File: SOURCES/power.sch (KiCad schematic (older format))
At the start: 1 part

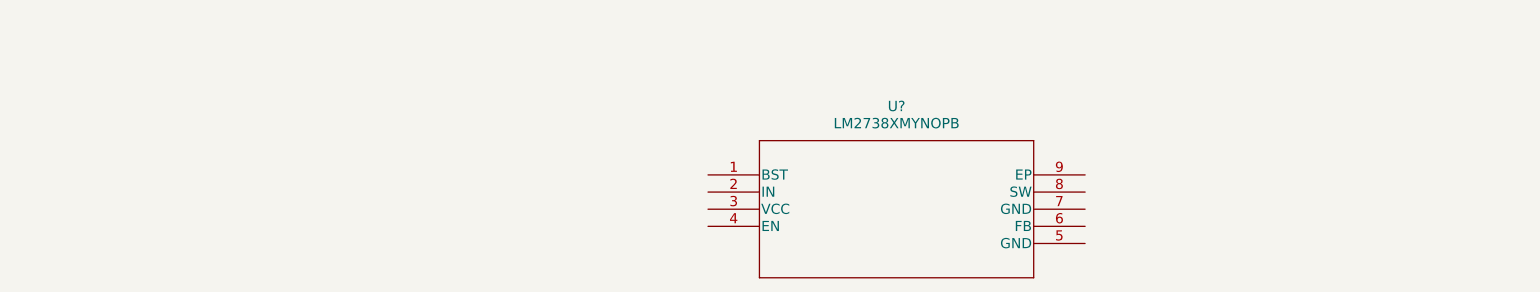
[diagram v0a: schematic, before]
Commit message: added power
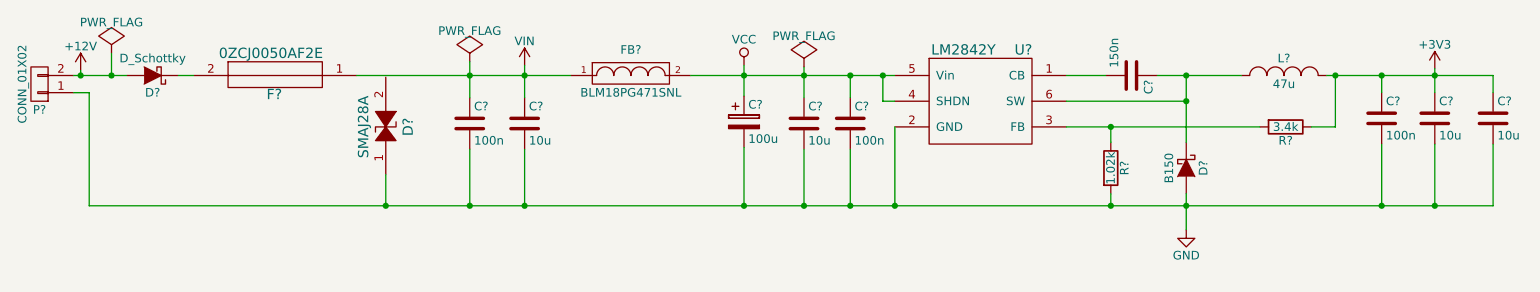
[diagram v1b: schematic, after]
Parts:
- removed U?: LM2738XMYNOPB, MUY08A, symbol LM2738XMYNOPB
- added C? (x3): 100n, symbol C
- added C? (x4): 10u, symbol C
- added C?: 100u, symbol CP
- added C?: 150n, symbol C
- added D?: D_Schottky, symbol D_Schottky
- added D?: SMAJ28A, symbol SMAJ28A
- added D?: B150, symbol D_Schottky
- added F?: 0ZCJ0050AF2E, symbol 0ZCJ0050AF2E
- added FB?: BLM18PG471SNL, symbol FILTER
- added L?: 47u, symbol Inductor
- added P?: CONN_01X02, symbol CONN_01X02
- added R?: 1.02k, symbol R
- added R?: 3.4k, symbol R
- added U?: LM2842Y, symbol LM284x
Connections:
- new net: C?.2, U?.1 (CB)
- new net: R?.1, R?.2, U?.3 (FB)
- new net: C?.1, D?.1 (K), L?.1, U?.6 (SW)
- new net: D?.1 (K), F?.2
- new net +12V: D?.2 (A), P?.2 (P2)
- new net +3V3: C?.1, C?.1, C?.1, L?.2, R?.1
- new net GND: C?.2, C?.2, C?.2, C?.2, C?.2, C?.2, C?.2, C?.2, D?.1, D?.2 (A), P?.1 (P1), R?.2, U?.2 (GND)
- new net VCC: C?.1, C?.1, C?.1, FB?.2, U?.4 (SHDN), U?.5 (Vin)
- new net VIN: C?.1, C?.1, F?.1, FB?.1
